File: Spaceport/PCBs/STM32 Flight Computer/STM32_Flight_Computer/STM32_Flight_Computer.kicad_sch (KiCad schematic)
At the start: 5 parts, among them U5 STM32H7A3ZIT6

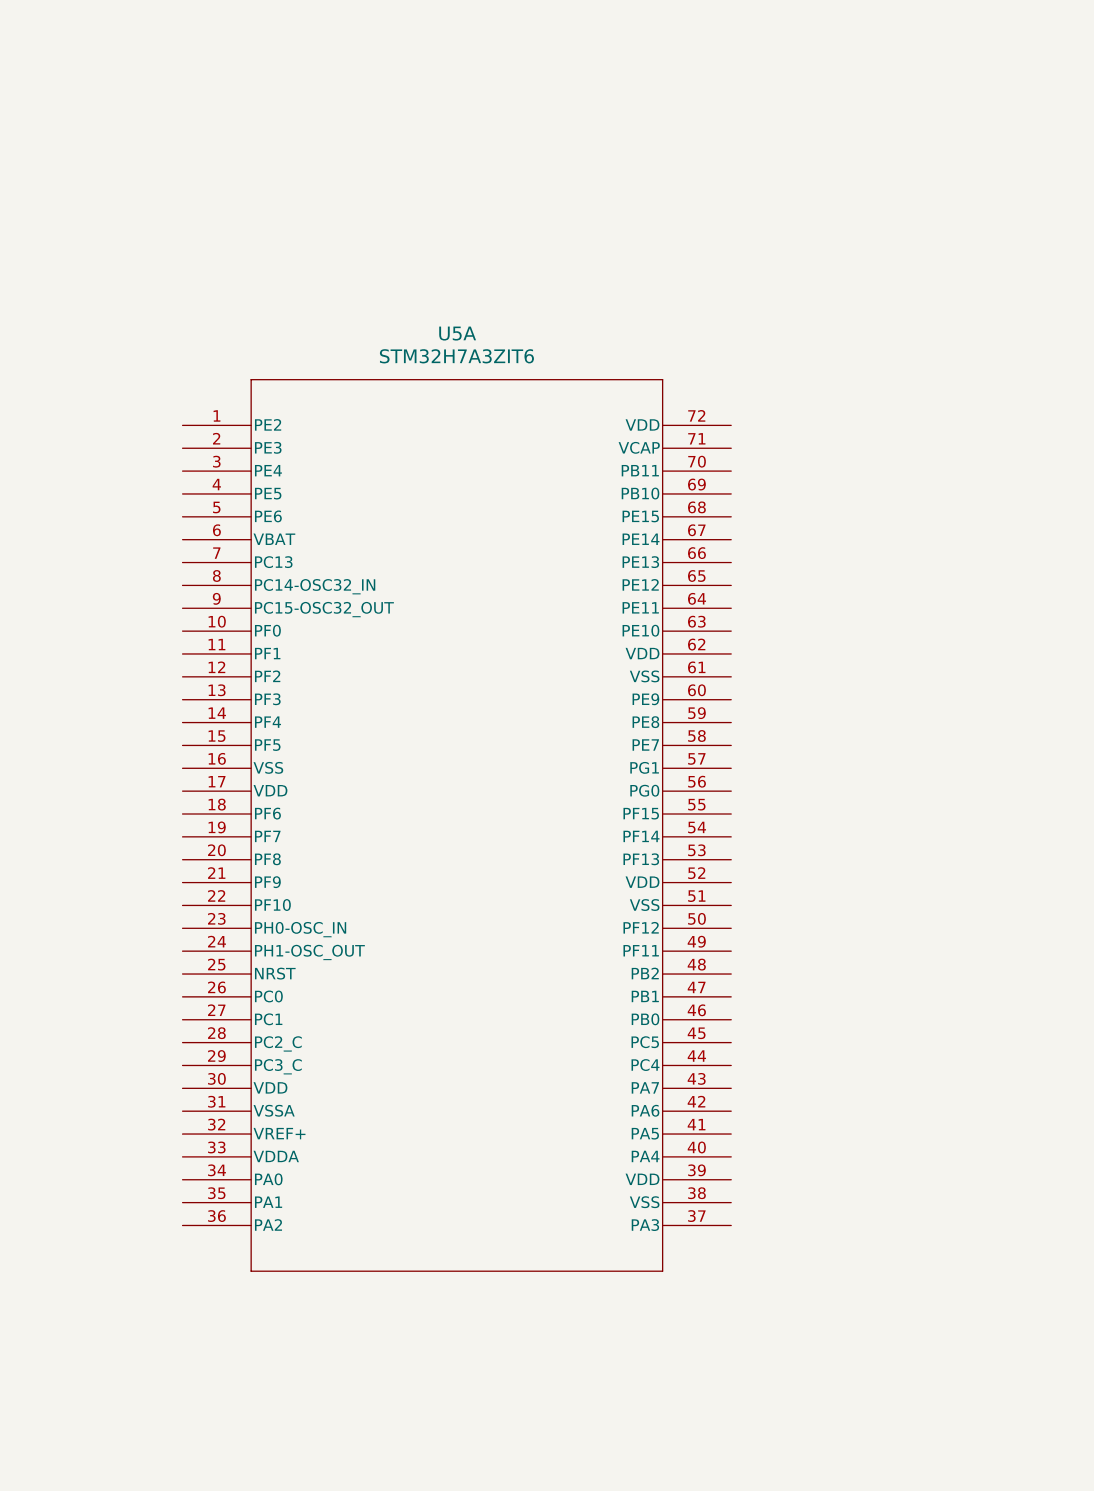
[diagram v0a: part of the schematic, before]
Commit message: Push
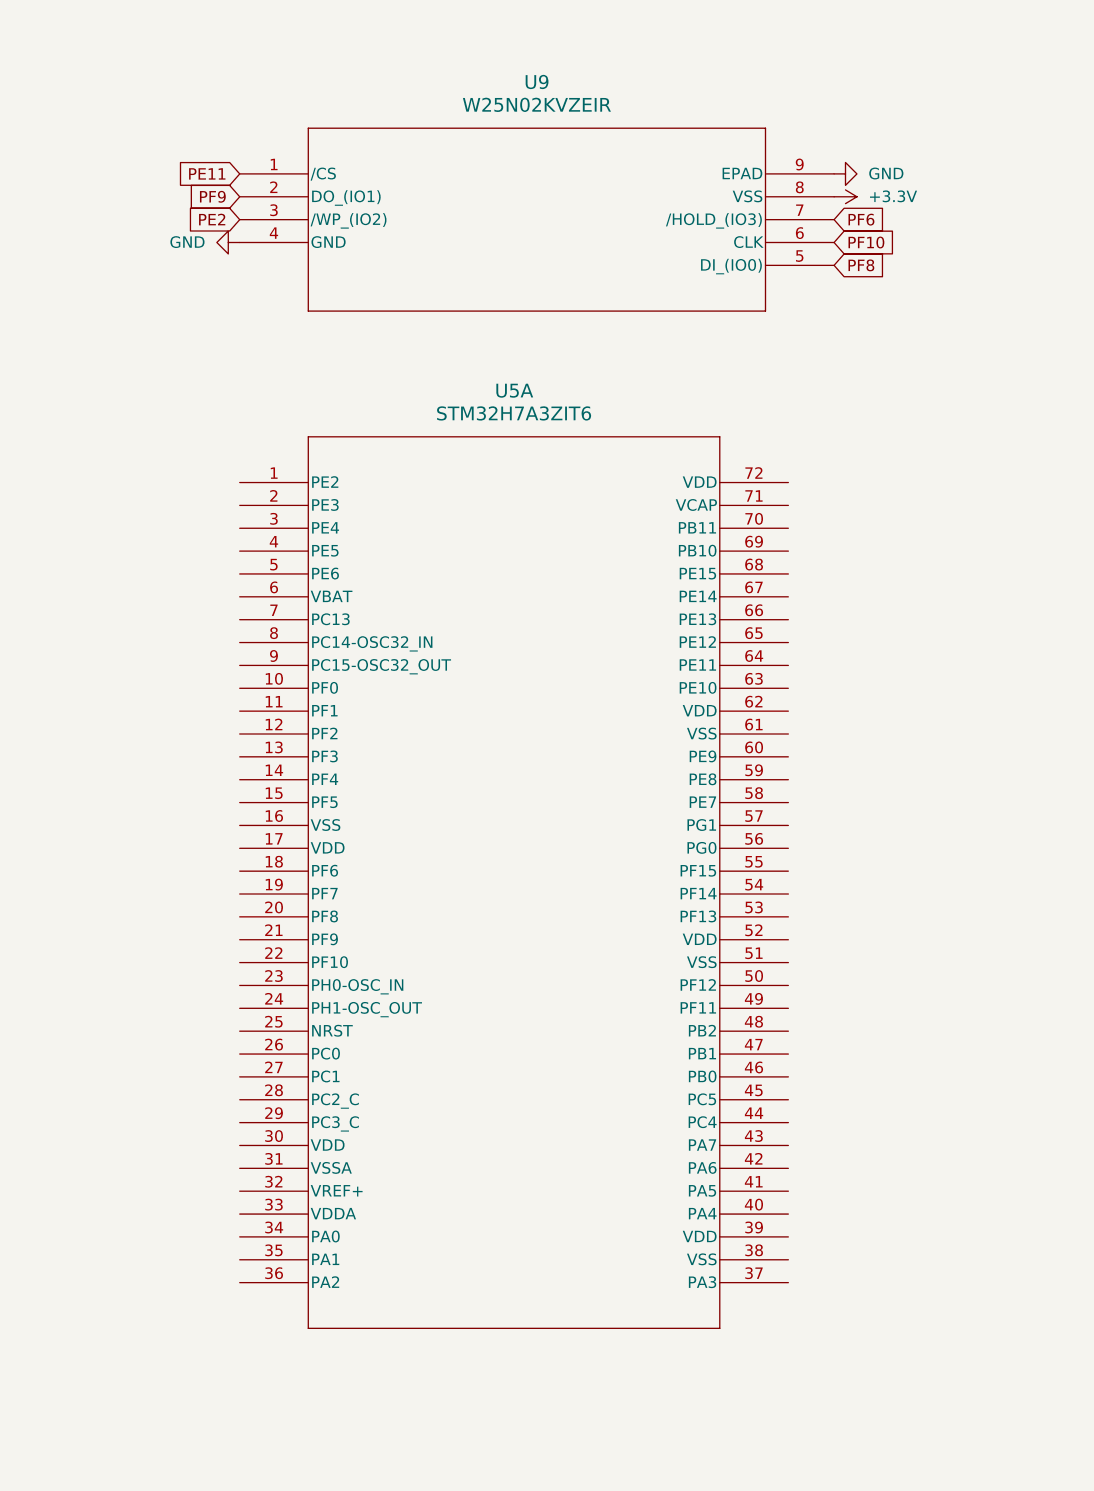
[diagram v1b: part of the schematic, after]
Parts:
- added U9: W25N02KVZEIR, SON_WSON8_ZE_WIN, symbol SRAD_AVIONICS:W25N02KVZEIR
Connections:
- new net +3.3V: U9.8 (VSS)
- new net GND: U9.4 (GND), U9.9 (EPAD)
- new net PE11: U9.1 (/CS)
- new net PE2: U9.3 (/WP_(IO2))
- new net PF10: U9.6 (CLK)
- new net PF6: U9.7 (/HOLD_(IO3))
- new net PF8: U9.5 (DI_(IO0))
- new net PF9: U9.2 (DO_(IO1))
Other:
- moved on the sheet: U5A

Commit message: Push after Schematic Review 5/5
- Updated STM32 symbol
- Configured I2C busses
- Updated DC caps to 100nF
- TODO add power system things
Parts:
- removed U5: STM32H7A3ZIT6, LQFP-144, symbol SRAD_AVIONICS:STM32H7A3ZIT6
- added C15: 100nF, symbol Device:C
- added U5: STM32H7A3ZITx, Package_QFP:LQFP-144_20x20mm_P0.5mm, symbol MCU_ST_STM32H7:STM32H7A3ZITx
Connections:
- net +3.3V: now also C15.2
- net GND: now also C15.1
- net PE11: now also U5.64 (PE11)
- net PE2: now also U5.1 (PE2)
- net PF10: now also U5.22 (PF10)
- net PF6: now also U5.18 (PF6)
- net PF8: now also U5.20 (PF8)
- net PF9: now also U5.21 (PF9)
- new net: U5.107 (VSS), U5.120 (VSS), U5.130 (VSS), U5.16 (VSS), U5.38 (VSS), U5.51 (VSS), U5.61 (VSS), U5.83 (VSS), U5.94 (VSS)
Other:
- note added: "I2C1"
- note added: "I2C2"
- moved on the sheet: H1, H2, H3, H4, U9
